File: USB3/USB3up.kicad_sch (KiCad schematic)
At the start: 5 parts

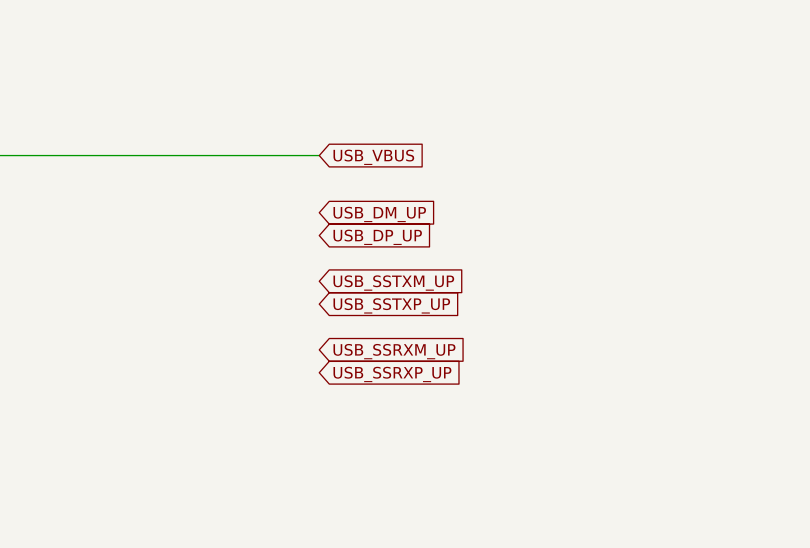
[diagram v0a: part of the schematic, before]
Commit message: usb3 work cont
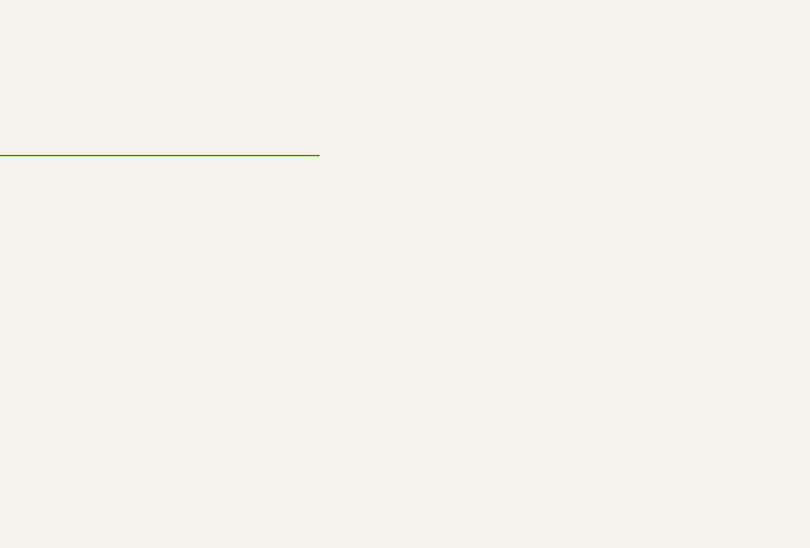
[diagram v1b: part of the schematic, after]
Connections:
- net USB_VBUS: no longer names the net of R22.2, R23.1
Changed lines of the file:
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@@
-		)
-	)
-	(global_label "USB_SSRXM_UP"
-		(shape input)
-		(at 217.17 59.69 0)
-		(fields_autoplaced yes)
-		(effects
-			(font
-				(size 1.27 1.27)
-			)
-			(justify left)
-		)
-		(property "Intersheetrefs" "${INTERSHEET_REFS}"
-			(at 234.8508 59.69 0)
-			(effects
-				(font
-					(size 1.27 1.27)
-				)
-				(justify left)
-				(hide yes)
-			)
-		)
-	)
-	(global_label "USB_DM_UP"
-		(shape input)
-		(at 217.17 44.45 0)
-		(fields_autoplaced yes)
-		(effects
-			(font
-				(size 1.27 1.27)
-			)
-			(justify left)
-		)
-		(property "Intersheetrefs" "${INTERSHEET_REFS}"
-			(at 231.2223 44.45 0)
-			(effects
-				(font
-					(size 1.27 1.27)
-				)
-				(justify left)
-				(hide yes)
-			)
-		)
-	)
-	(global_label "USB_SSTXM_UP"
-		(shape input)
-		(at 217.17 52.07 0)
-		(fields_autoplaced yes)
-		(effects
-			(font
-				(size 1.27 1.27)
-			)
-			(justify left)
-		)
-		(property "Intersheetrefs" "${INTERSHEET_REFS}"
-			(at 234.5484 52.07 0)
-			(effects
-				(font
-					(size 1.27 1.27)
-				)
-				(justify left)
-				(hide yes)
-			)
 		)
 	)
@@
 				(hide yes)
 			)
-		)
-	)
-	(global_label "USB_SSRXP_UP"
-		(shape input)
-		(at 217.17 62.23 0)
-		(fields_autoplaced yes)
-		(effects
-			(font
-				(size 1.27 1.27)
-			)
-			(justify left)
-		)
-		(property "Intersheetrefs" "${INTERSHEET_REFS}"
-			(at 234.6694 62.23 0)
-			(effects
-				(font
-					(size 1.27 1.27)
-				)
-				(justify left)
-				(hide yes)
-			)
-		)
-	)
-	(global_label "USB_SSTXP_UP"
-		(shape input)
-		(at 217.17 54.61 0)
-		(fields_autoplaced yes)
-		(effects
-			(font
-				(size 1.27 1.27)
-			)
-			(justify left)
-		)
-		(property "Intersheetrefs" "${INTERSHEET_REFS}"
-			(at 234.367 54.61 0)
-			(effects
-				(font
-					(size 1.27 1.27)
-				)
-				(justify left)
-				(hide yes)
-			)
-		)
-	)
-	(global_label "USB_VBUS"
-		(shape input)
-		(at 217.17 38.1 0)
-		(fields_autoplaced yes)
-		(effects
-			(font
-				(size 1.27 1.27)
-			)
-			(justify left)
-		)
-		(property "Intersheetrefs" "${INTERSHEET_REFS}"
-			(at 229.8314 38.1 0)
-			(effects
-				(font
-					(size 1.27 1.27)
-				)
-				(justify left)
-				(hide yes)
-			)
-		)
-	)
-	(global_label "USB_DP_UP"
-		(shape input)
-		(at 217.17 46.99 0)
-		(fields_autoplaced yes)
-		(effects
-			(font
-				(size 1.27 1.27)
-			)
-			(justify left)
-		)
-		(property "Intersheetrefs" "${INTERSHEET_REFS}"
-			(at 231.0409 46.99 0)
-			(effects
-				(font
-					(size 1.27 1.27)
-				)
-				(justify left)
-				(hide yes)
-			)
